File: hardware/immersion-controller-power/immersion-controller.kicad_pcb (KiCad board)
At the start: 2 copper layers, 130.5 x 73.6 mm, 31 parts, among them J1 MCU, J6 HEATER-E, J7 HEATER-N, J8 HEATER-L, J9 MAINS_IN, K3 HEATER-BOTTOM, K4 HEATER-TOP, Q4 2N3904, Q5 2N3904, U10 PC817, U6 AMS1117-3.3, U9 PC817

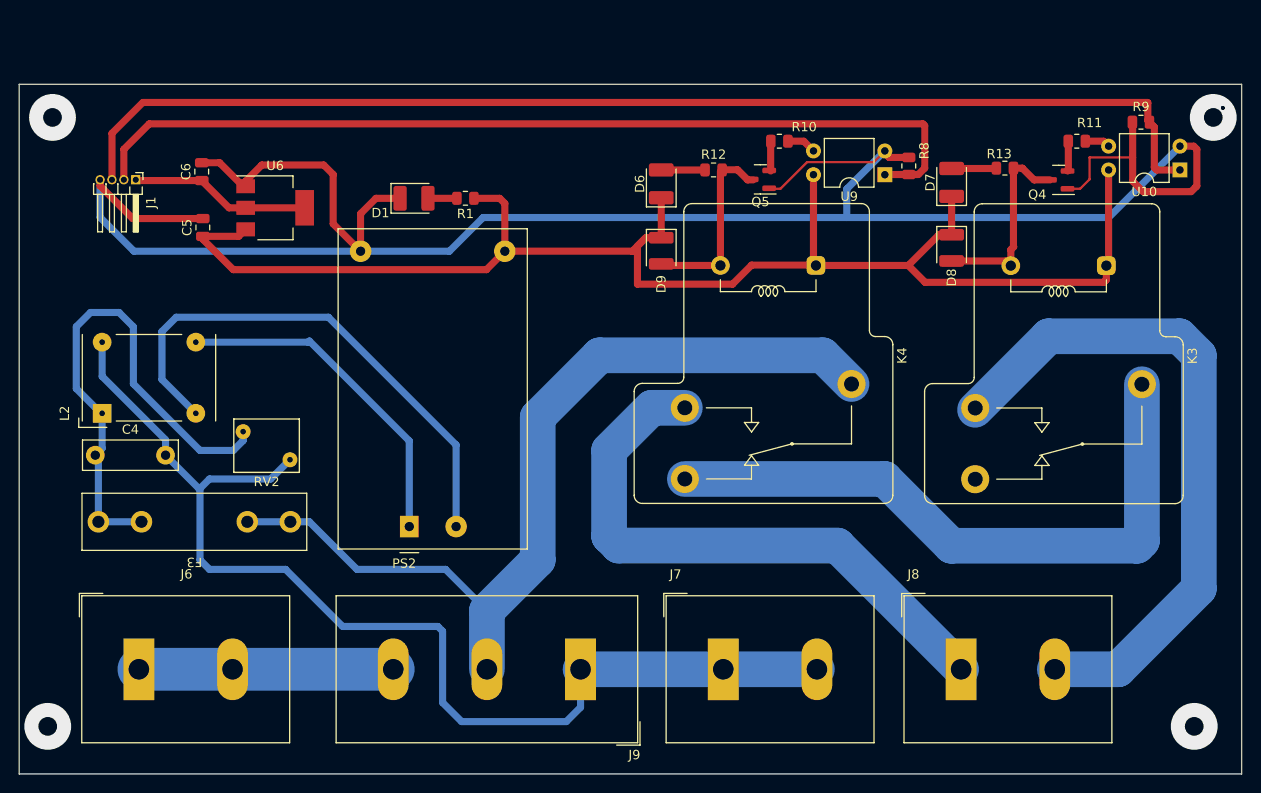
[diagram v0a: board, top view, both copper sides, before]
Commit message: debugged prototype
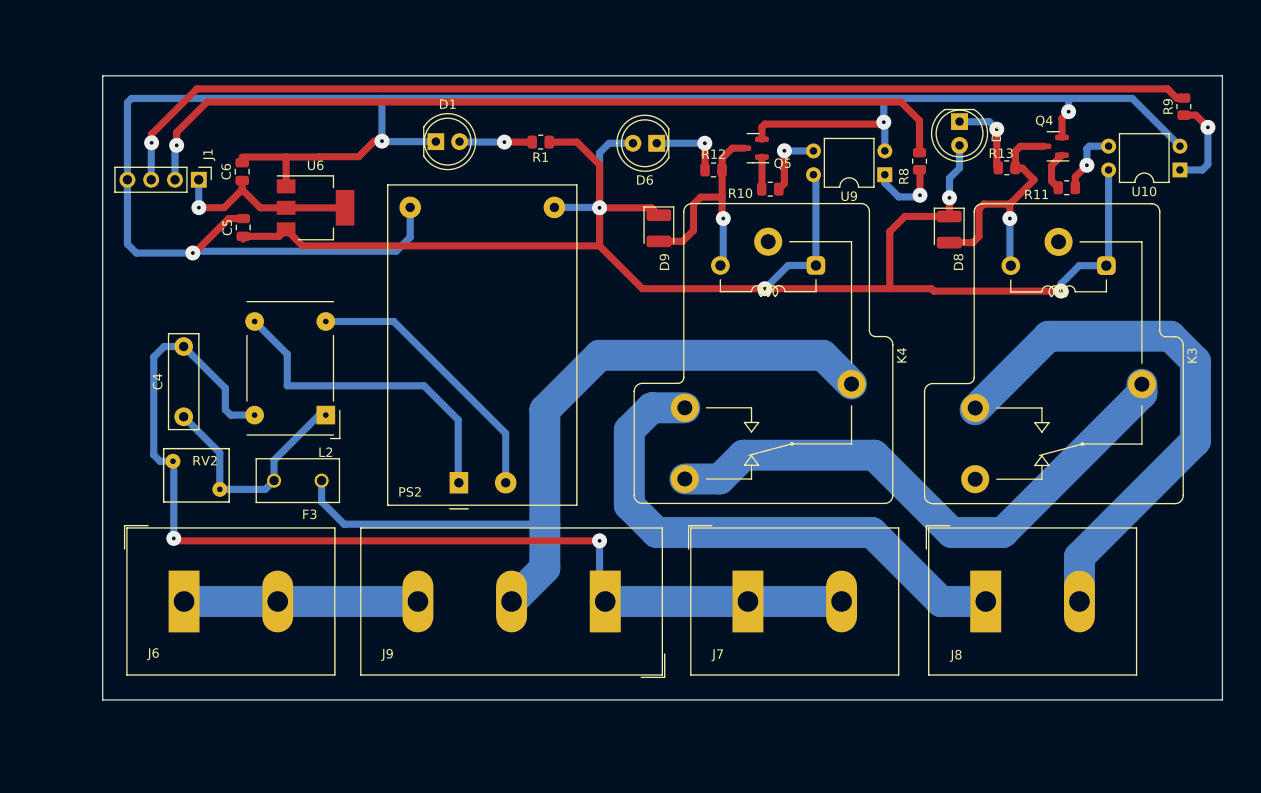
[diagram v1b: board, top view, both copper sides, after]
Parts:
- D1, D6, D7: footprint Diode_SMD:D_1210_3225Metric_Pad1.42x2.65mm_HandSolder -> LED_THT:LED_D5.0mm_Clear
- F3: value 1A -> 500 mA; footprint Fuse:Fuseholder_Littelfuse_100_series_5x20mm -> TE5:FUSE_BK_PCE-5-R
- J1: footprint Connector_PinHeader_1.27mm:PinHeader_1x04_P1.27mm_Horizontal -> Connector_PinHeader_2.54mm:PinHeader_1x04_P2.54mm_Vertical
- K3, K4: footprint Relay_THT:Relay_SPDT_RAYEX-L90S -> Relay_THT:Relay_SPDT_RAYEX-L90
- Q4, Q5: value 2N3904 -> MMBT3904
- moved L2 23.9 mm to (41.4, 158.3), turned to 180 degrees
- moved C4 10.3 mm to (26.2, 158.5), turned to 90 degrees
- moved R1 10.0 mm to (64.3, 129.1)
- moved J6 8.70 mm to (26.2, 178.2)
- moved J7 7.70 mm to (86.5, 178.2)
- moved J8 7.70 mm to (111.9, 178.2)
- moved J9 7.70 mm to (71.2, 178.2)
- moved PS2 7.07 mm to (55.6, 165.5)
- moved J1 6.73 mm to (27.8, 133.1)
- moved RV2 6.65 mm to (30.1, 166.2), turned to 180 degrees
- moved D7 6.55 mm to (109.0, 126.9), turned to -90 degrees
- moved D1 6.48 mm to (53.1, 129.1)
- moved R10 5.21 mm to (88.8, 134.2)
- moved R11 5.08 mm to (120.5, 134.0)
- moved R9 4.87 mm to (133.0, 125.3), turned to 90 degrees
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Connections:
- D6 pad 1: +5V -> Net-(D6-K)
- D6 pad 2: Net-(D6-A) -> +5V
- D7 pad 1: +5V -> Net-(D7-K)
- D7 pad 2: Net-(D7-A) -> +5V
- K4 pad 12: Net-(K3-Pad11) -> Net-(K3-Pad11B)
- Q4 pad 1: GND -> Net-(Q4-B)
- Q4 pad 2: Net-(Q4-B) -> GND
- Q5 pad 1: GND -> Net-(Q5-B)
- Q5 pad 2: Net-(Q5-B) -> GND
- R12 pad 1: Net-(D6-A) -> Net-(D6-K)
- R13 pad 1: Net-(D7-A) -> Net-(D7-K)
- R8 pad 1: GND -> Net-(R8-Pad1)
- R9 pad 1: GND -> Net-(R9-Pad1)
- U10 pad 1: RELAY_BOTTOM -> Net-(R9-Pad1)
- U9 pad 1: RELAY_TOP -> Net-(R8-Pad1)
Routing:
- net Net-(K3-Pad11): track 68.7 -> 0.00 mm
- net Net-(K3-Pad11B): track 0.00 -> 60.4 mm
- net Net-(C4-Pad1): track 56.6 -> 25.2 mm
- net Net-(PS2-AC/N): track 56.6 -> 29.4 mm
- net +5V: track 158.6 -> 182.6 mm, vias 0 -> 4
- net Net-(J8-Pin_2): track 71.8 -> 58.7 mm
- net MAINSIN_L: track 96.2 -> 85.5 mm
- net Net-(R9-Pad1): track 0.00 -> 10.3 mm, vias 0 -> 1
- net RELAY_BOTTOM: track 127.0 -> 117.5 mm, vias 0 -> 1
- net RELAY_TOP: track 99.1 -> 90.1 mm, vias 0 -> 1
- net Net-(D7-K): track 0.00 -> 8.68 mm, vias 0 -> 1
- net Net-(R8-Pad1): track 0.00 -> 8.10 mm, vias 0 -> 1
- net MAINSIN_N: track 120.7 -> 112.7 mm, vias 0 -> 2
- net Net-(D6-K): track 0.00 -> 7.99 mm, vias 0 -> 1
- net Net-(D8-A): track 22.0 -> 29.0 mm, vias 0 -> 1
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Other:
- board size 130.5 x 73.6 mm -> 119.6 x 66.6 mm

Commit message: Initial Prototype results
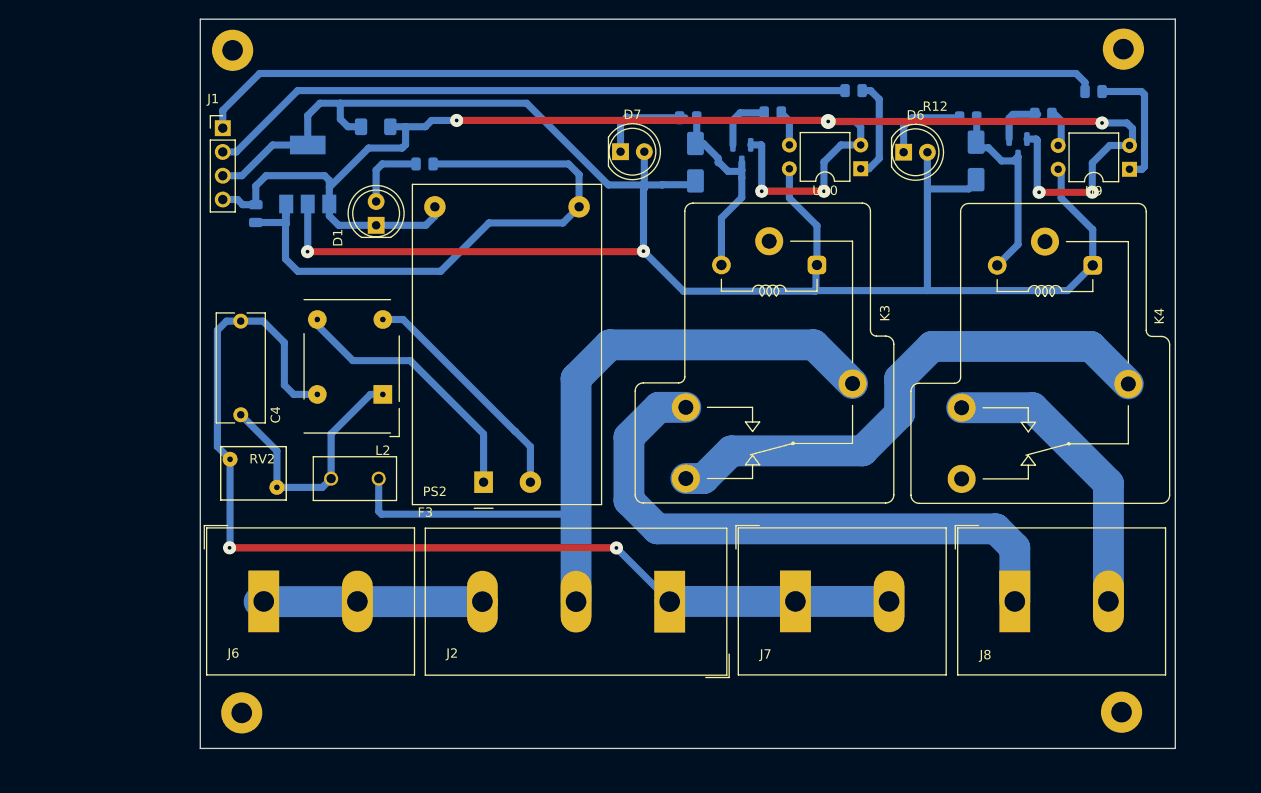
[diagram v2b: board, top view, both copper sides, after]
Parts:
- removed J9: MAINS_IN, TerminalBlock_Dinkle:TerminalBlock_Dinkle_DT-55-B01X-03_P10.00mm
- added J2: MAINS_IN, TerminalBlock_Dinkle:TerminalBlock_Dinkle_DT-55-B01X-03_P10.00mm, F.Cu at (78.1, 178.2)
- added REF**: MountingHole_2.2mm_M2_Pad, MountingHole:MountingHole_2.2mm_M2_Pad, F.Cu at (126.3, 190.0)
- added REF**: MountingHole_2.2mm_M2_Pad, MountingHole:MountingHole_2.2mm_M2_Pad, F.Cu at (31.4, 119.3)
- added REF**: MountingHole_2.2mm_M2_Pad, MountingHole:MountingHole_2.2mm_M2_Pad, F.Cu at (32.4, 190.1)
- added REF**: MountingHole_2.2mm_M2_Pad, MountingHole:MountingHole_2.2mm_M2_Pad, F.Cu at (126.5, 119.2)
- C4: footprint Capacitor_THT:C_Rect_L10.0mm_W3.0mm_P7.50mm_MKS4 -> Capacitor_THT:C_Rect_L11.5mm_W5.0mm_P10.00mm_MKT
- C5, Q4, Q5, R1, R10, R11, R12, R13, R8, R9, U6: moved to B.Cu
- C6: footprint Capacitor_SMD:C_0805_2012Metric -> Capacitor_SMD:C_1206_3216Metric_Pad1.33x1.80mm_HandSolder; moved to B.Cu
- D8, D9: value 1N4007 -> US1M; footprint Diode_SMD:D_1210_3225Metric -> Diode_SMD:D_SMA; moved to B.Cu
- moved D7 36.3 mm to (72.8, 130.2), turned to 0 degrees
- moved R9 35.3 mm to (97.7, 123.6), turned to 180 degrees
- moved D9 34.6 mm to (110.8, 131.1), turned to 90 degrees
- moved R13 34.4 mm to (80.1, 126.5)
- moved U10 34.1 mm to (98.5, 132.0)
- moved Q4 33.3 mm to (85.8, 130.4), turned to -90 degrees
- moved R11 32.4 mm to (89.1, 126.0)
- moved K3 30.9 mm to (88.7, 139.7)
- moved R10 30.2 mm to (118.0, 126.2)
- moved K4 29.6 mm to (118.2, 139.8)
- moved Q5 28.3 mm to (115.3, 129.7), turned to -90 degrees
- moved D8 28.0 mm to (80.8, 131.3), turned to 90 degrees
- moved R12 27.7 mm to (110.0, 126.5)
- moved D6 26.4 mm to (103.1, 130.2), turned to 0 degrees
- moved U9 26.1 mm to (127.2, 132.0)
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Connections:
- D6 pad 2: +5V -> +3.3V
- D7 pad 2: +5V -> +3.3V
- D8 pad 1: +5V -> +3.3V
- D9 pad 1: +5V -> +3.3V
- J1 pad 1: +3.3V -> RELAY_TOP
- J1 pad 2: RELAY_TOP -> RELAY_BOTTOM
- J1 pad 3: RELAY_BOTTOM -> +3.3V
- K3 pad 11B: Net-(K3-Pad11B) -> MAINSIN_L
- K3 pad 12: unconnected-(K3-Pad12) -> Net-(K3-Pad12)
- K3 pad 14: Net-(J8-Pin_2) -> Net-(J8-Pin_1)
- K3 pad A1: +5V -> +3.3V
- K4 pad 11B: MAINSIN_L -> Net-(K3-Pad12)
- K4 pad 12: Net-(K3-Pad11B) -> unconnected-(K4-Pad12)
- K4 pad 14: Net-(J8-Pin_1) -> Net-(J8-Pin_2)
- K4 pad A1: +5V -> +3.3V
- U10 pad 4: +5V -> +3.3V
- U9 pad 4: +5V -> +3.3V
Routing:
- net +3.3V: track 21.2 -> 212.2 mm, vias 1 -> 2
- net +5V: track 182.6 -> 64.5 mm, vias 4 -> 0
- net Net-(K3-Pad11B): track 60.4 -> 0.00 mm
- net Net-(K3-Pad12): track 0.00 -> 56.9 mm
- net GND: track 225.8 -> 171.9 mm, vias 4 -> 7
- net RELAY_BOTTOM: track 117.5 -> 69.2 mm, vias 1 -> 0
- net Net-(J8-Pin_2): track 58.7 -> 31.6 mm
- net Net-(D8-A): track 29.0 -> 21.2 mm, vias 1 -> 0
- net RELAY_TOP: track 90.1 -> 97.0 mm, vias 1 -> 0
- net Net-(PS2-AC/L): track 34.8 -> 28.6 mm
- net Net-(J8-Pin_1): track 57.2 -> 63.2 mm
- net Net-(R8-Pad1): track 8.10 -> 13.8 mm, vias 1 -> 0
- net Net-(PS2-AC/N): track 29.4 -> 25.2 mm
- net Net-(D9-A): track 25.1 -> 21.0 mm, vias 1 -> 0
- net Net-(R10-Pad1): track 7.46 -> 3.61 mm, vias 1 -> 0
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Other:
- board size 119.6 x 66.6 mm -> 104.1 x 77.9 mm
